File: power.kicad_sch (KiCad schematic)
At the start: 22 parts, among them U1 74HC04, U10 74HC08, U11 74HC74, U12 74HC4050, U13 74HC4050, U2 74HC00, U4 74HC11, U8 74HC04, U9 74HC74

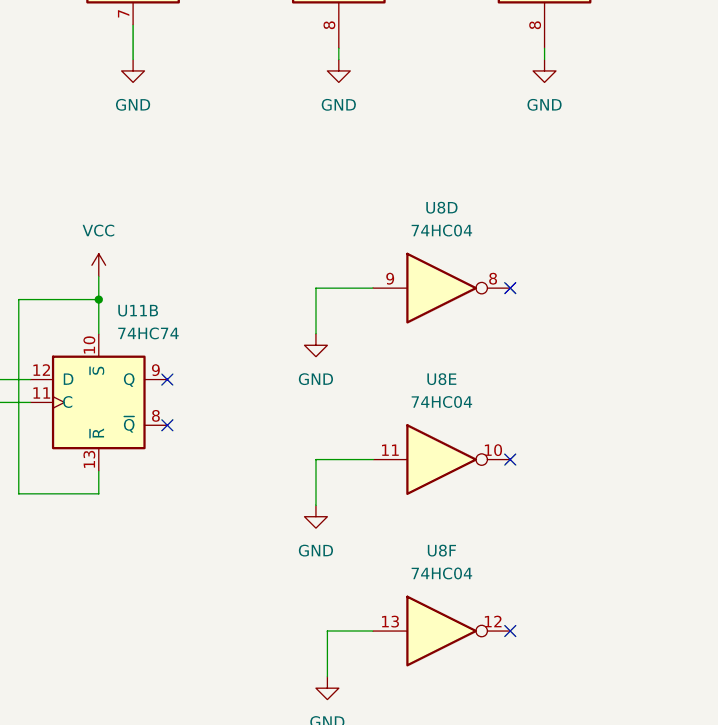
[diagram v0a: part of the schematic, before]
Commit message: Update to Rev B.
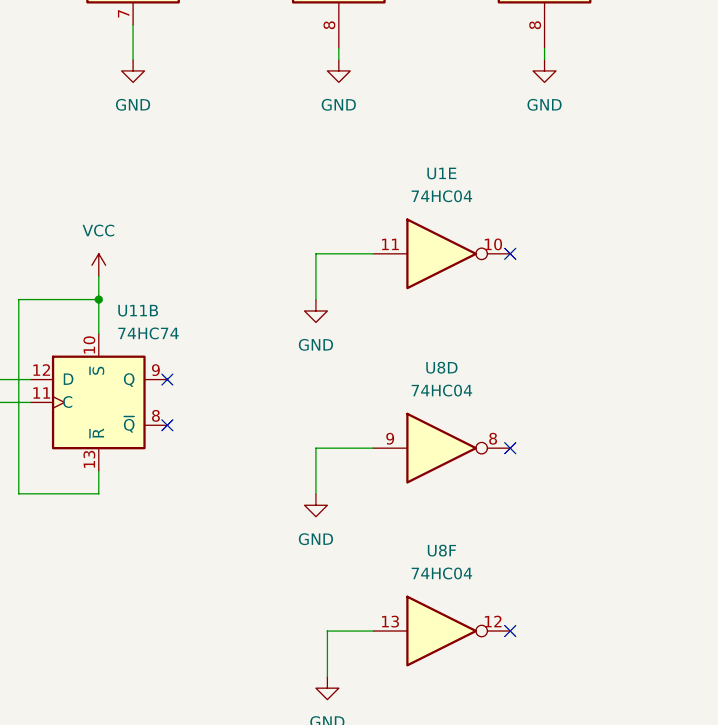
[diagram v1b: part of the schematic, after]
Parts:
- removed unit 5 of U8
- added unit 5 of U1
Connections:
- net GND: now also U1.11
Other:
- moved on the sheet: U8D
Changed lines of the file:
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@@
   (junction (at 57.15 157.48) (diameter 0) (color 0 0 0 0)
   )
-  (no_connect (at 224.79 96.52))
+  (no_connect (at 224.79 114.3))
   (no_connect (at 224.79 134.62))
-  (no_connect (at 224.79 115.57))
+  (no_connect (at 224.79 92.71))
   (no_connect (at 186.69 106.68))
   (no_connect (at 186.69 111.76))
@@
     (stroke (width 0) (type default) (color 0 0 0 0))
   )
-  (wire (pts (xy 203.2 115.57) (xy 209.55 115.57))
+  (wire (pts (xy 203.2 92.71) (xy 209.55 92.71))
     (stroke (width 0) (type default) (color 0 0 0 0))
   )
@@
     (stroke (width 0) (type default) (color 0 0 0 0))
   )
-  (wire (pts (xy 203.2 120.65) (xy 203.2 115.57))
+  (wire (pts (xy 203.2 97.79) (xy 203.2 92.71))
     (stroke (width 0) (type default) (color 0 0 0 0))
   )
@@
     (stroke (width 0) (type default) (color 0 0 0 0))
   )
-  (wire (pts (xy 203.2 101.6) (xy 203.2 96.52))
+  (wire (pts (xy 203.2 119.38) (xy 203.2 114.3))
     (stroke (width 0) (type default) (color 0 0 0 0))
   )
@@
     (stroke (width 0) (type default) (color 0 0 0 0))
   )
-  (wire (pts (xy 203.2 96.52) (xy 209.55 96.52))
+  (wire (pts (xy 203.2 114.3) (xy 209.55 114.3))
     (stroke (width 0) (type default) (color 0 0 0 0))
   )
@@
     (pin "7")
   )
-  (symbol (lib_id "74xx:74HC04") (at 217.17 115.57 0) (unit 5)
-    (in_bom yes) (on_board yes) (fields_autoplaced)
-    (property "Reference" "U8" (id 0) (at 217.17 106.68 0))
-    (property "Value" "74HC04" (id 1) (at 217.17 109.22 0))
-    (property "Footprint" "Package_DIP:DIP-14_W7.62mm_Socket" (id 2) (at 217.17 115.57 0)
-      (effects (font (size 1.27 1.27)) hide)
-    )
-    (property "Datasheet" "https://assets.nexperia.com/documents/data-sheet/74HC_HCT04.pdf" (id 3) (at 217.17 115.57 0)
-      (effects (font (size 1.27 1.27)) hide)
-    )
-    (pin "1")
-    (pin "2")
-    (pin "3")
-    (pin "4")
-    (pin "5")
-    (pin "6")
-    (pin "8")
-    (pin "9")
-    (pin "10")
-    (pin "11")
-    (pin "12")
-    (pin "13")
-    (pin "14")
-    (pin "7")
-  )
   (symbol (lib_id "Device:C") (at 43.18 110.49 180) (unit 1)
     (in_bom yes) (on_board yes) (fields_autoplaced)
@@
     (pin "2")
   )
+  (symbol (lib_id "74xx:74HC04") (at 217.17 92.71 0) (unit 5)
+    (in_bom yes) (on_board yes) (fields_autoplaced)
+    (property "Reference" "U1" (id 0) (at 217.17 83.82 0))
+    (property "Value" "74HC04" (id 1) (at 217.17 86.36 0))
+    (property "Footprint" "Package_DIP:DIP-14_W7.62mm_Socket" (id 2) (at 217.17 92.71 0)
+      (effects (font (size 1.27 1.27)) hide)
+    )
+    (property "Datasheet" "https://assets.nexperia.com/documents/data-sheet/74HC_HCT04.pdf" (id 3) (at 217.17 92.71 0)
+      (effects (font (size 1.27 1.27)) hide)
+    )
+    (pin "1")
+    (pin "2")
+    (pin "3")
+    (pin "4")
+    (pin "5")
+    (pin "6")
+    (pin "8")
+    (pin "9")
+    (pin "10")
+    (pin "11")
+    (pin "12")
+    (pin "13")
+    (pin "14")
+    (pin "7")
+  )
   (symbol (lib_id "power:GND") (at 160.02 71.12 0) (unit 1)
     (in_bom yes) (on_board yes) (fields_autoplaced)
@@
     (pin "1")
   )
-  (symbol (lib_id "74xx:74HC04") (at 217.17 96.52 0) (unit 4)
-    (in_bom yes) (on_board yes) (fields_autoplaced)
-    (property "Reference" "U8" (id 0) (at 217.17 87.63 0))
-    (property "Value" "74HC04" (id 1) (at 217.17 90.17 0))
-    (property "Footprint" "Package_DIP:DIP-14_W7.62mm_Socket" (id 2) (at 217.17 96.52 0)
-      (effects (font (size 1.27 1.27)) hide)
-    )
-    (property "Datasheet" "https://assets.nexperia.com/documents/data-sheet/74HC_HCT04.pdf" (id 3) (at 217.17 96.52 0)
+  (symbol (lib_id "74xx:74HC04") (at 217.17 114.3 0) (unit 4)
+    (in_bom yes) (on_board yes) (fields_autoplaced)
+    (property "Reference" "U8" (id 0) (at 217.17 105.41 0))
+    (property "Value" "74HC04" (id 1) (at 217.17 107.95 0))
+    (property "Footprint" "Package_DIP:DIP-14_W7.62mm_Socket" (id 2) (at 217.17 114.3 0)
+      (effects (font (size 1.27 1.27)) hide)
+    )
+    (property "Datasheet" "https://assets.nexperia.com/documents/data-sheet/74HC_HCT04.pdf" (id 3) (at 217.17 114.3 0)
       (effects (font (size 1.27 1.27)) hide)
     )
@@
     (pin "1")
   )
-  (symbol (lib_id "power:GND") (at 203.2 120.65 0) (unit 1)
-    (in_bom yes) (on_board yes) (fields_autoplaced)
-    (property "Reference" "#PWR047" (id 0) (at 203.2 127 0)
-      (effects (font (size 1.27 1.27)) hide)
-    )
-    (property "Value" "GND" (id 1) (at 203.2 125.73 0))
-    (property "Footprint" "" (id 2) (at 203.2 120.65 0)
-      (effects (font (size 1.27 1.27)) hide)
-    )
-    (property "Datasheet" "" (id 3) (at 203.2 120.65 0)
+  (symbol (lib_id "power:GND") (at 203.2 97.79 0) (unit 1)
+    (in_bom yes) (on_board yes) (fields_autoplaced)
+    (property "Reference" "#PWR047" (id 0) (at 203.2 104.14 0)
+      (effects (font (size 1.27 1.27)) hide)
+    )
+    (property "Value" "GND" (id 1) (at 203.2 102.87 0))
+    (property "Footprint" "" (id 2) (at 203.2 97.79 0)
+      (effects (font (size 1.27 1.27)) hide)
+    )
+    (property "Datasheet" "" (id 3) (at 203.2 97.79 0)
       (effects (font (size 1.27 1.27)) hide)
     )
@@
     (pin "7")
   )
-  (symbol (lib_id "power:GND") (at 203.2 101.6 0) (unit 1)
-    (in_bom yes) (on_board yes) (fields_autoplaced)
-    (property "Reference" "#PWR046" (id 0) (at 203.2 107.95 0)
-      (effects (font (size 1.27 1.27)) hide)
-    )
-    (property "Value" "GND" (id 1) (at 203.2 106.68 0))
-    (property "Footprint" "" (id 2) (at 203.2 101.6 0)
-      (effects (font (size 1.27 1.27)) hide)
-    )
-    (property "Datasheet" "" (id 3) (at 203.2 101.6 0)
-      (effects (font (size 1.27 1.27)) hide)
-    )
+  (symbol (lib_id "power:GND") (at 203.2 119.38 0) (unit 1)
+    (in_bom yes) (on_board yes) (fields_autoplaced)
+    (property "Reference" "#PWR046" (id 0) (at 203.2 125.73 0)
+      (effects (font (size 1.27 1.27)) hide)
+    )
+    (property "Value" "GND" (id 1) (at 203.2 124.46 0))
+    (property "Footprint" "" (id 2) (at 203.2 119.38 0)
+      (effects (font (size 1.27 1.27)) hide)
+    )
+    (property "Datasheet" "" (id 3) (at 203.2 119.38 0)
+      (effects (font (size 1.27 1.27)) hide)
+    )
